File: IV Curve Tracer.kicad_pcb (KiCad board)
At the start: 2 copper layers, 80 x 85 mm, 87 parts, among them J1 9V Supply, J2 Solar Array, J3 CAN_In, J4 CAN_Out, Q1 IRF100P218XKMA1, Q2 IRF100P218XKMA1, SW1 SW_Push, SW2 A20303RNCG, U1 MCU_Nucleo_L432KC, U2 INA210, U3 LT1215, U4 MAX680ESA+, U5 ADM3055E, U6 CDSOT23-T24CAN

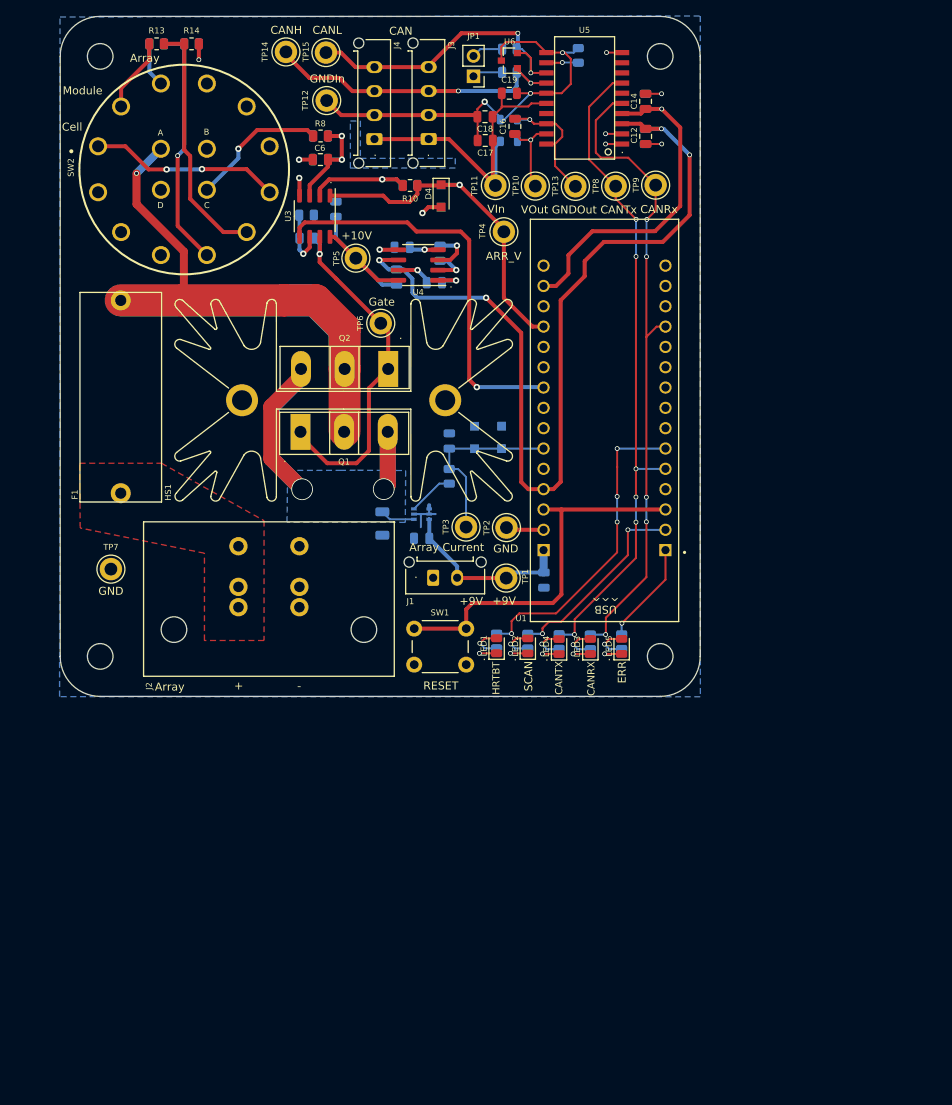
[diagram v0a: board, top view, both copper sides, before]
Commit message: v1.2.0 rc with new layout.
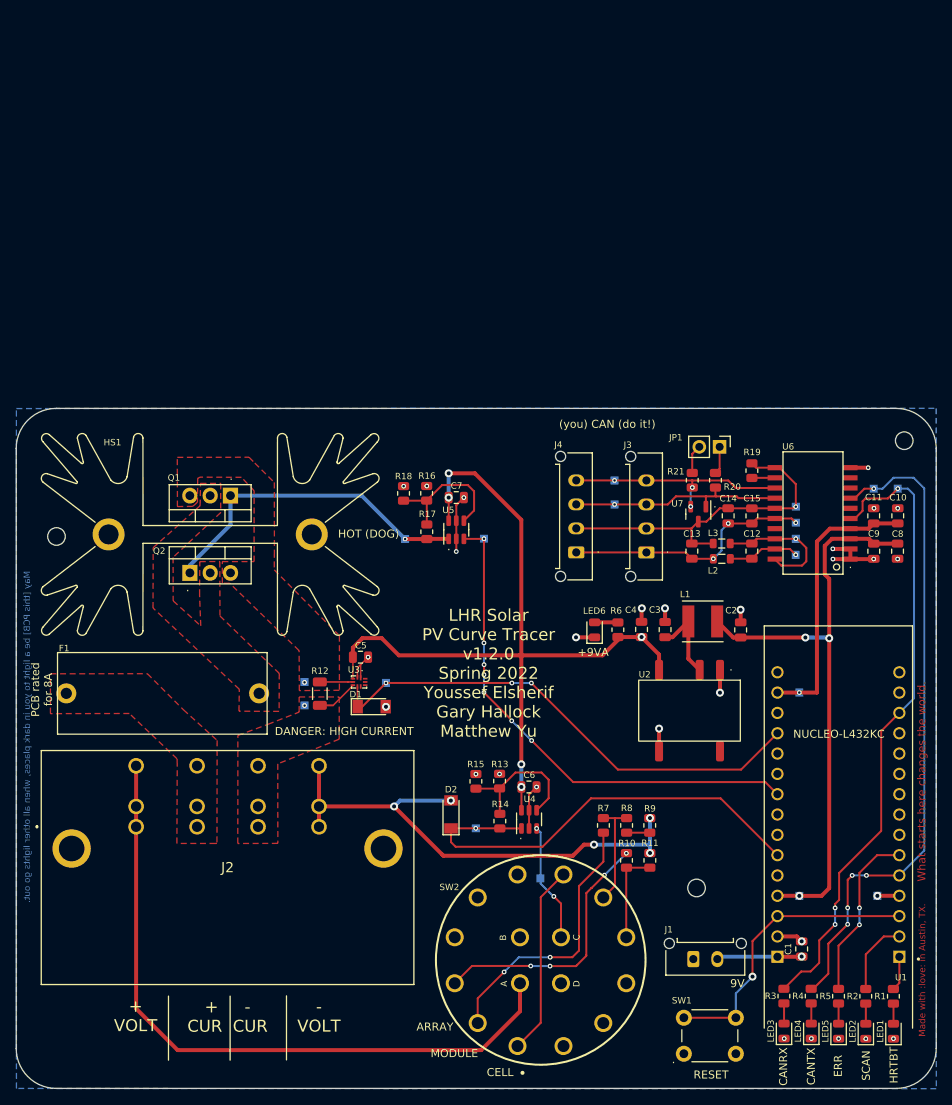
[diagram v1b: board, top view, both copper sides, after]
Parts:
- removed C16: .22uF, Capacitor_SMD:C_0805_2012Metric
- removed C17: 10uF, Capacitor_SMD:C_0805_2012Metric
- removed C18: .1uF, Capacitor_SMD:C_0805_2012Metric
- removed C19: .01uF, Capacitor_SMD:C_0805_2012Metric
- removed D3: 3.9V Zener, Diode_SMD:D_SOD-123F
- removed D4: Diode, Diode_SMD:D_SOD-123F
- removed the G*** at (88.2, 47.2)
- removed H4: MountingHole, MountingHole:MountingHole_3.2mm_M3
- added L3: 1.8kOhm, Inductor_SMD:L_0805_2012Metric, F.Cu at (102.7, 85.9)
- added LED6: 9V (Green), LED_SMD:LED_0805_2012Metric, F.Cu at (86.8, 96.7)
- added R20: 60.4, Resistor_SMD:R_0805_2012Metric, F.Cu at (101.9, 78.0)
- added R21: 60.4, Resistor_SMD:R_0805_2012Metric, F.Cu at (99.0, 78.0)
- added REF**: KiCad-Logo2_5mm_SilkScreen, Symbol:KiCad-Logo2_5mm_SilkScreen, B.Cu at (117.2, 122.5)
- added REF**: ESD-Logo_8.9x8mm_SilkScreen, Symbol:ESD-Logo_8.9x8mm_SilkScreen, B.Cu at (117.3, 114.9)
- added TP16: CAN_ISO_Vin, TestPoint:TestPoint_Pad_1.0x1.0mm, B.Cu at (112.0, 83.3)
- added TP17: CAN_ISO_GndIn, TestPoint:TestPoint_Pad_1.0x1.0mm, B.Cu at (112.0, 81.3)
- added TP18: CAN_ISO_GndOut, TestPoint:TestPoint_Pad_1.0x1.0mm, B.Cu at (112.0, 85.3)
- added TP19: CAN_H, TestPoint:TestPoint_Pad_1.0x1.0mm, B.Cu at (89.3, 81.0)
- added TP20: CAN_L, TestPoint:TestPoint_Pad_1.0x1.0mm, B.Cu at (89.3, 78.0)
- added U7: CDSOT23-T24CAN, Package_TO_SOT_SMD:SOT-23, F.Cu at (99.8, 82.2)
- C1, C5, C7: value 0.1uF -> 100nF; moved to F.Cu
- C10, C9: value 4.7uF -> 100nF; moved to F.Cu
- C11: value 4.7uF -> 10nF; moved to F.Cu
- C12: value 10uF -> 220nF
- C13: value .1uF -> 10uF; moved to F.Cu
- C14: value .1uF -> 100nF
- C15: value .01uF -> 10nF; moved to F.Cu
- C2: value 0.1uF -> 4.7uF; moved to F.Cu
- C3: value 1uF -> 4.7uF; moved to F.Cu
- C4: value 1uF -> 2.2uF; moved to F.Cu
- C6: value 0.01uF -> 100nF
- C8: value 4.7uF -> 10uF; moved to F.Cu
- D1: value 3.9V Zener -> 3.3V Zener; footprint Diode_SMD:D_SOD-123F -> Diode_SMD:D_MiniMELF; moved to F.Cu
- D2: value Diode -> 3.3V Zener; footprint Diode_SMD:D_SOD-123F -> Diode_SMD:D_MiniMELF; moved to F.Cu
- H1, H2, H3: footprint MountingHole:MountingHole_3.2mm_M3 -> MountingHole:MountingHole_2.2mm_M2
- J2: value Solar Array -> 1720819; footprint IV Curve Tracer:PhoenixContact_PowerCombicon5_GF_2x7.62mm -> IV Curve Tracer:1720819
- JP1: value Termination Resistors -> Jumper
- L1: value 1.8kH -> 6.8uH; footprint Inductor_SMD:L_0805_2012Metric -> Inductor_SMD:L_Taiyo-Yuden_NR-50xx; moved to F.Cu
- L2: value 1.8kH -> 1.8kOhm; moved to F.Cu
- Q1, Q2: footprint Package_TO_SOT_THT:TO-247-3_Vertical -> Package_TO_SOT_THT:TO-220-3_Vertical
- R1, R2, R3, R4, R5: moved to F.Cu
- R10: value 1k -> 100k
- R11: value 4k -> 1k; moved to F.Cu
- R12: value 1k -> 2m; footprint Resistor_SMD:R_0805_2012Metric -> Resistor_SMD:R_1206_3216Metric; moved to F.Cu
- R13: value 56.6k -> 1k
- R14: value 10k -> 1k
- R15: value 132k -> 1k; moved to F.Cu
- R16: value 2k -> 1k; moved to F.Cu
- R17: value 0 -> 1k; moved to F.Cu
- R18: value 60 -> 1k; moved to F.Cu
- R19: value 60 -> 0; moved to F.Cu
- R6: value 2m -> 330; footprint Resistor_SMD:R_1206_3216Metric -> Resistor_SMD:R_0805_2012Metric; moved to F.Cu
- R7: value 1.7k -> 6.8k; moved to F.Cu
- R8: value 10k -> 1.5k
- R9: value 1k -> 220; moved to F.Cu
- TP1: footprint TestPoint:TestPoint_Keystone_5005-5009_Compact -> TestPoint:TestPoint_Pad_1.0x1.0mm; moved to B.Cu
- TP10: value CAN_ISO_Vout -> Array Voltage; footprint TestPoint:TestPoint_Keystone_5005-5009_Compact -> TestPoint:TestPoint_Pad_1.0x1.0mm; moved to B.Cu
- TP11: value CAN_ISO_Vin -> Pre Gate Voltage; footprint TestPoint:TestPoint_Keystone_5005-5009_Compact -> TestPoint:TestPoint_Pad_1.0x1.0mm; moved to B.Cu
- TP12: value CAN_ISO_GndIn -> Gate Voltage; footprint TestPoint:TestPoint_Keystone_5005-5009_Compact -> TestPoint:TestPoint_Pad_1.0x1.0mm; moved to B.Cu
- TP13: value CAN_ISO_GndOut -> CAN_Tx; footprint TestPoint:TestPoint_Keystone_5005-5009_Compact -> TestPoint:TestPoint_Pad_1.0x1.0mm; moved to B.Cu
- TP14: value CAN_H -> CAN_Rx; footprint TestPoint:TestPoint_Keystone_5005-5009_Compact -> TestPoint:TestPoint_Pad_1.0x1.0mm; moved to B.Cu
- TP15: value CAN_L -> CAN_ISO_Vout; footprint TestPoint:TestPoint_Keystone_5005-5009_Compact -> TestPoint:TestPoint_Pad_1.0x1.0mm; moved to B.Cu
- TP2: value GND -> 5V; footprint TestPoint:TestPoint_Keystone_5005-5009_Compact -> TestPoint:TestPoint_Pad_1.0x1.0mm; moved to B.Cu
- TP3: value Array_I -> 3V3; footprint TestPoint:TestPoint_Keystone_5005-5009_Compact -> TestPoint:TestPoint_Pad_1.0x1.0mm; moved to B.Cu
- TP4: value Array Voltage -> GND; footprint TestPoint:TestPoint_Keystone_5005-5009_Compact -> TestPoint:TestPoint_Pad_1.0x1.0mm; moved to B.Cu
- TP5: value +10V -> 9VA; footprint TestPoint:TestPoint_Keystone_5005-5009_Compact -> TestPoint:TestPoint_Pad_1.0x1.0mm; moved to B.Cu
- TP6: value Gate -> Pre Array Current +; footprint TestPoint:TestPoint_Keystone_5005-5009_Compact -> TestPoint:TestPoint_Pad_1.0x1.0mm; moved to B.Cu
- TP7: value GND -> Pre Array Current -; footprint TestPoint:TestPoint_Keystone_5005-5009_Compact -> TestPoint:TestPoint_Pad_1.0x1.0mm; moved to B.Cu
- TP8: value CAN_Tx -> Array Current; footprint TestPoint:TestPoint_Keystone_5005-5009_Compact -> TestPoint:TestPoint_Pad_1.0x1.0mm; moved to B.Cu
- TP9: value CAN_Rx -> Pre Array Voltage; footprint TestPoint:TestPoint_Keystone_5005-5009_Compact -> TestPoint:TestPoint_Pad_1.0x1.0mm; moved to B.Cu
- U2: value INA210 -> IES01_PDS1; footprint IV Curve Tracer:SC70-6 -> IV Curve Tracer:IES01_PDS1; moved to F.Cu
- U3: value LT1215 -> INA210; footprint Package_SO:SO-8_3.9x4.9mm_P1.27mm -> Package_DFN_QFN:UQFN-10_1.4x1.8mm_P0.4mm
- U4: value MAX680ESA+ -> MAX40075; footprint Package_SO:SOIC-8_3.9x4.9mm_P1.27mm -> Package_TO_SOT_SMD:SOT-23-6
- U5: value ADM3055E -> MAX40075; footprint IV Curve Tracer:ADM3055EBRIZ -> Package_TO_SOT_SMD:SOT-23-6
- U6: value CDSOT23-T24CAN -> ADM3055E; footprint Package_TO_SOT_SMD:SOT-23 -> IV Curve Tracer:ADM3055EBRIZ
- moved SW2 108.5 mm to (80.0, 138.0), turned to -90 degrees
- moved R14 104.5 mm to (75.0, 120.6), turned to 90 degrees
- moved R13 101.6 mm to (74.9, 115.6), turned to 90 degrees
- moved R15 100.4 mm to (72.0, 115.6), turned to 90 degrees
- moved TP4 95.2 mm to (122.2, 129.9)
- moved R8 94.3 mm to (90.8, 121.1), turned to -90 degrees
- moved TP14 94.0 mm to (124.7, 79.0), turned to 0 degrees
- moved R11 88.8 mm to (93.7, 125.5), turned to 90 degrees
- moved R10 88.6 mm to (90.8, 125.5), turned to -90 degrees
- moved TP9 87.8 mm to (80.0, 127.7), turned to 0 degrees
- moved TP15 86.0 mm to (111.9, 87.3)
- moved R9 85.4 mm to (93.7, 121.1), turned to 90 degrees
- moved C6 82.6 mm to (78.6, 116.3)
- moved TP10 80.6 mm to (72.0, 121.5), turned to 0 degrees
- moved H3 80.0 mm to (99.5, 128.9)
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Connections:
- C10 pad 1: +10V -> GND
- C10 pad 2: +5V -> +3V3
- C11 pad 1: GND -> +3V3
- C11 pad 2: -10V -> GND
- C12 pad 1: +5V -> Net-(C12-Pad1)
- C12 pad 2: GND -> Net-(C12-Pad2)
- C13 pad 1: +5V -> Net-(C13-Pad1)
- C13 pad 2: GND -> Net-(C13-Pad2)
- C14 pad 1: +3V3 -> Net-(C13-Pad2)
- C14 pad 2: GND -> Net-(C13-Pad1)
- C15 pad 1: +3V3 -> Net-(C13-Pad1)
- C15 pad 2: GND -> Net-(C13-Pad2)
- C2 pad 1: GND -> +5V
- C2 pad 2: +9V -> GND
- C3 pad 1: /Array_Current -> Net-(C3-Pad1)
- C4 pad 1: Net-(C4-Pad1) -> +9VA
- C5 pad 1: Net-(C4-Pad1) -> GND
- C5 pad 2: GND -> +9VA
- C6 pad 1: Net-(C4-Pad1) -> GND
- C6 pad 2: GND -> +9VA
- C7 pad 2: +10V -> +9VA
- C8 pad 1: Net-(C8-Pad1) -> +5V
- C8 pad 2: Net-(C8-Pad2) -> GND
- C9 pad 1: Net-(C9-Pad1) -> GND
- C9 pad 2: Net-(C9-Pad2) -> +5V
- D2 pad 1: /Array_Current -> /Array_Voltage
- J2 pad 1: Net-(F1-Pad2) -> Net-(J2-Pad1)
- J2 pad 2: GND -> Net-(J2-Pad1)
- J3 pad 1: Net-(C17-Pad1) -> Net-(C13-Pad1)
- J3 pad 2: Net-(C17-Pad2) -> Net-(C13-Pad2)
- J4 pad 1: Net-(C17-Pad1) -> Net-(C13-Pad1)
- J4 pad 2: Net-(C17-Pad2) -> Net-(C13-Pad2)
- L1 pad 1: Net-(C17-Pad1) -> +5V
- L1 pad 2: Net-(C16-Pad1) -> Net-(C3-Pad1)
- L2 pad 1: Net-(C17-Pad2) -> Net-(C13-Pad1)
- L2 pad 2: Net-(C16-Pad2) -> Net-(C12-Pad1)
- Q1 pad 3: /+Current_Sense -> Net-(Q1-Pad3)
- Q2 pad 3: /+Current_Sense -> Net-(Q1-Pad3)
- R10 pad 1: /Array_Voltage -> Net-(R10-Pad1)
- R11 pad 1: /Gate -> Net-(R10-Pad2)
- R11 pad 2: Net-(R11-Pad2) -> GND
- R12 pad 1: Net-(R11-Pad2) -> Net-(J2-Pad7)
- R12 pad 2: GND -> Net-(Q1-Pad3)
- R13 pad 2: Net-(R13-Pad2) -> GND
- R14 pad 1: Net-(R13-Pad2) -> /Array_Voltage
- R14 pad 2: GND -> Net-(R13-Pad1)
- R15 pad 1: Net-(R15-Pad1) -> Net-(R13-Pad1)
- R15 pad 2: Net-(R15-Pad2) -> GND
- R16 pad 1: Net-(R15-Pad2) -> Net-(R16-Pad1)
- R17 pad 1: Net-(C17-Pad2) -> /Gate
- R17 pad 2: Net-(R17-Pad2) -> Net-(R16-Pad1)
- R18 pad 1: Net-(JP1-Pad1) -> Net-(R16-Pad1)
- R18 pad 2: Net-(J3-Pad3) -> GND
- R19 pad 1: Net-(J3-Pad4) -> Net-(R19-Pad1)
- R19 pad 2: Net-(JP1-Pad2) -> Net-(C13-Pad2)
- R6 pad 1: GND -> +9VA
- R6 pad 2: /+Current_Sense -> Net-(LED6-Pad2)
- R7 pad 1: /Array_Current -> Net-(R7-Pad1)
- R8 pad 1: /Voltage_Sense -> Net-(R7-Pad2)
- R8 pad 2: Net-(C4-Pad1) -> Net-(R8-Pad2)
- R9 pad 1: Net-(R10-Pad2) -> Net-(R8-Pad2)
- SW2 pad 13: Net-(F1-Pad1) -> Net-(J2-Pad1)
- SW2 pad 2: Net-(R13-Pad1) -> Net-(R7-Pad1)
- SW2 pad 3: Net-(R15-Pad1) -> Net-(R10-Pad1)
- SW2 pad 8: Net-(R13-Pad2) -> Net-(R7-Pad2)
- SW2 pad 9: Net-(R15-Pad2) -> Net-(R10-Pad2)
- TP10 pad 1: Net-(C16-Pad1) -> /Array_Voltage
- TP11 pad 1: Net-(C17-Pad1) -> /DAC_Control
- TP12 pad 1: Net-(C17-Pad2) -> /Gate
- TP13 pad 1: Net-(C16-Pad2) -> /CAN_Tx
- TP14 pad 1: Net-(J3-Pad3) -> /CAN_Rx
- TP15 pad 1: Net-(J3-Pad4) -> Net-(C12-Pad1)
- TP2 pad 1: GND -> +5V
- TP3 pad 1: /Array_Current -> +3V3
- TP4 pad 1: /Array_Voltage -> GND
- TP5 pad 1: +10V -> +9VA
- TP6 pad 1: /Gate -> Net-(Q1-Pad3)
- TP7 pad 1: GND -> Net-(J2-Pad7)
- TP8 pad 1: /CAN_Tx -> /Array_Current
- TP9 pad 1: /CAN_Rx -> /Voltage_Sense
- U1 pad 1: /Error -> /Heartbeat
- U1 pad 10: Net-(U1-Pad10) -> unconnected-(U1-Pad10)
- U1 pad 11: Net-(U1-Pad11) -> unconnected-(U1-Pad11)
- U1 pad 12: /CAN_Rx -> unconnected-(U1-Pad12)
- U1 pad 13: Net-(U1-Pad13) -> /CAN_Rx
- U1 pad 14: Net-(U1-Pad14) -> unconnected-(U1-Pad14)
- U1 pad 15: Net-(U1-Pad15) -> unconnected-(U1-Pad15)
- U1 pad 16: Net-(U1-Pad16) -> unconnected-(U1-Pad16)
- U1 pad 18: Net-(U1-Pad18) -> unconnected-(U1-Pad18)
- U1 pad 19: /Array_Voltage -> /Array_Current
- U1 pad 20: Net-(U1-Pad20) -> unconnected-(U1-Pad20)
- U1 pad 21: Net-(U1-Pad21) -> unconnected-(U1-Pad21)
- U1 pad 23: Net-(U1-Pad23) -> unconnected-(U1-Pad23)
- U1 pad 24: Net-(U1-Pad24) -> unconnected-(U1-Pad24)
- U1 pad 25: /Array_Current -> /Array_Voltage
- U1 pad 26: Net-(U1-Pad26) -> unconnected-(U1-Pad26)
- U1 pad 6: /Heartbeat -> /Error
- U1 pad 7: Net-(U1-Pad7) -> unconnected-(U1-Pad7)
- U1 pad 8: Net-(U1-Pad8) -> unconnected-(U1-Pad8)
- U1 pad 9: Net-(U1-Pad9) -> unconnected-(U1-Pad9)
- U2 pad 2: GND -> Net-(C3-Pad1)
- U2 pad 4: /+Current_Sense -> +9VA
- U3 pad 1: /Array_Voltage -> GND
- U3 pad 2: Net-(R10-Pad2) -> GND
- U3 pad 3: Net-(C4-Pad1) -> +9VA
- U3 pad 4: GND -> Net-(Q1-Pad3)
- U3 pad 5: /DAC_Control -> Net-(J2-Pad7)
- U3 pad 6: Net-(R11-Pad2) -> /Array_Current
- U3 pad 7: /Gate -> (no net)
- U3 pad 8: +10V -> (no net)
- U4 pad 1: Net-(C9-Pad1) -> /Array_Voltage
- U4 pad 2: Net-(C8-Pad2) -> GND
- U4 pad 3: Net-(C8-Pad1) -> /Voltage_Sense
- U4 pad 4: -10V -> Net-(R13-Pad1)
- U4 pad 6: +5V -> +9VA
- U5 pad 1: GND -> /Gate
- U5 pad 3: +5V -> /DAC_Control
- U5 pad 4: +3V3 -> Net-(R16-Pad1)
- U5 pad 5: /CAN_Rx -> GND
- U5 pad 6: Net-(U5-Pad6) -> +9VA
- U6 pad 1: Net-(J3-Pad3) -> GND
- U6 pad 2: Net-(J3-Pad4) -> GND
- U6 pad 3: Net-(C17-Pad2) -> +5V
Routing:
- net +9VA: track 0.00 -> 101.5 mm, vias 0 -> 5
- net Net-(F1-Pad1): track 99.5 -> 0.00 mm, vias 1 -> 0
- net Net-(J2-Pad1): track 0.00 -> 86.0 mm
- net GND: track 42.5 -> 111.1 mm, vias 15 -> 34
- net Net-(C17-Pad2): track 57.2 -> 0.00 mm, vias 3 -> 0
- net /+Current_Sense: track 55.4 -> 0.00 mm, vias 2 -> 0
- net Net-(C13-Pad2): track 0.00 -> 41.9 mm, vias 0 -> 1
- net Net-(C17-Pad1): track 41.2 -> 0.00 mm
- net /Array_Current: track 23.1 -> 62.5 mm, vias 0 -> 3
- net +5V: track 113.0 -> 74.5 mm, vias 4 -> 3
- net /Heartbeat: track 39.2 -> 4.34 mm, vias 4 -> 0
- net Net-(R7-Pad1): track 0.00 -> 34.2 mm, vias 0 -> 2
- net Net-(R10-Pad1): track 0.00 -> 32.8 mm, vias 0 -> 4
- net Net-(C13-Pad1): track 0.00 -> 31.6 mm, vias 0 -> 3
- net Net-(R13-Pad2): track 31.0 -> 0.00 mm
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- added copper zone on F.Cu, net Net-(F1-Pad1)
- added copper zone on F.Cu, net Net-(J2-Pad7)
- added copper zone on F.Cu, net Net-(Q1-Pad3)
- removed copper zone on B.Cu, net /+Current_Sense
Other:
- board size 80 x 85 mm -> 115 x 85 mm
- net class Default removed
- board text added: "(you) CAN (do it!)"
- board text added: "+ - CUR CUR"
- board text added: "+ VOLT"
- board text added: "+3V3"
- board text added: "+5V"
- board text added: "+9VA"
- board text added: "- VOLT"
- board text added: "9V"
- board text added: "<GND_TIE"
- board text added: "ARRAY"
- board text added: "ARR_CURRENT"
- board text added: "ARR_CURRENT+"
- board text added: "ARR_CURRENT-"
- board text added: "ARR_VOLTAGE"
- board text added: "CAN MCU signals (RX, TX) are single ended. Do not closely couple or risk crosstalk."
- board text added: "CELL"
- board text added: "Contact: matthewjkyu@gmail.com"
- board text added: "DAC_CONTROL"
- board text added: "DANGER: HIGH CURRENT"
- board text added: "GATE"
- board text added: "HOT (DOG)"
- board text added: "ISO_GNDIN"
- board text added: "ISO_GNDOUT"
- board text added: "ISO_VIN"
- board text added: "ISO_VOUT"
- board text added: "LHR Solar PV Curve Tracer v1.2.0 Spring 2022 Youssef Elsherif Gary Hallock Matthew Yu"
- board text added: "MODULE"
- board text added: "Made with :love: in Austin, TX."
- board text added: "May [this PCB] be a light to you in dark places, when all other lights go out."
- board text added: "NUCLEO-L432KC"
- board text added: "PCB rated for 8A"
- board text added: "Under the STM32."
- board text added: "VOLTAGE_SENSE"
- board text added: "What starts here changes the world."
- board text removed: "+"
- board text removed: "+10V"
- board text removed: "-"
- board text removed: "ARR_V"
- board text removed: "Array"
- board text removed: "Array Current"
- board text removed: "CAN"
- board text removed: "CANRx"
- board text removed: "CANTx"
- board text removed: "Cell"
- board text removed: "GNDIn"
- board text removed: "GNDOut"
- board text removed: "Gate"
- board text removed: "Module"
- board text removed: "Separating high power fluctuations from digital and analog signals."
- board text removed: "This looks a little odd, but hopefully it protects the analog signal a little bit from power and digital fluctuations."
- board text removed: "U2"
- board text removed: "USB ^^^"
- board text removed: "UTSVT - Array PV Curve Tracer Board v1.1 Fall 2020 Youssef Elsherif Gary Hallock Matthew Yu"
- board text removed: "VIn"
- board text removed: "VOut"
- board text removed: "We get pretty tight here."
- board text removed: "Wide trace to reduce resistance and voltage drop as much as possible"
